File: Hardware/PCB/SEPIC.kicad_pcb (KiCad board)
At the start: 2 copper layers, 33.6 x 35.9 mm, 27 parts, among them Q1 IRF7807, U1 LM3478MA

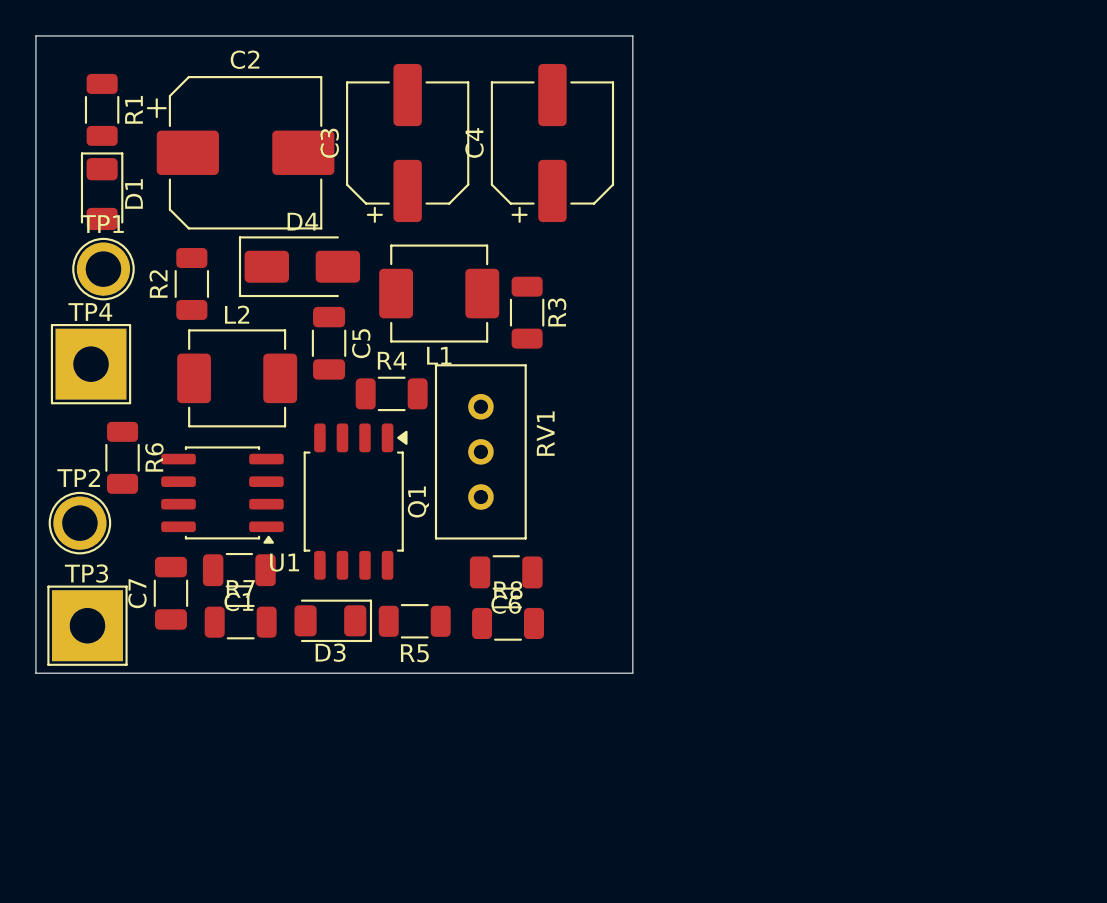
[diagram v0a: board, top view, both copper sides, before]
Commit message: Finished PCB layout
A few minor adjustments still need to be made
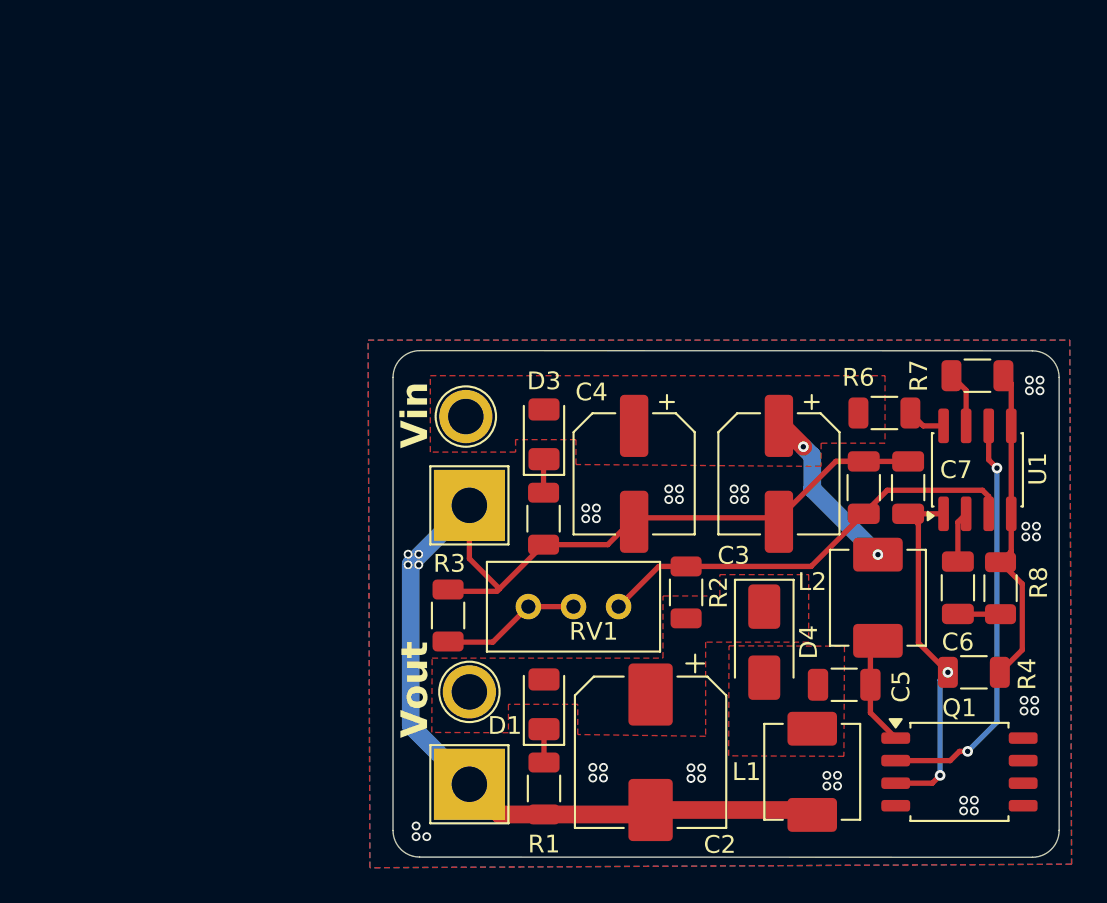
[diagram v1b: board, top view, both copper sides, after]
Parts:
- added G***: LOGO, Logo_footprint:Logo_10_6, B.Cu at (124.3, 65.1)
- added G***: LOGO, Logo_footprint:Logo_15_15, B.Cu at (110.5, 65.2)
- moved R1 45.6 mm to (99.9, 75.8), turned to 90 degrees
- moved R7 43.7 mm to (124.3, 52.6), turned to 180 degrees
- moved R6 43.0 mm to (119.1, 54.7), turned to 180 degrees
- moved U1 42.5 mm to (124.3, 57.9), turned to 90 degrees
- moved C7 41.9 mm to (120.4, 58.9), turned to -90 degrees
- moved C2 40.7 mm to (105.9, 73.8), turned to -90 degrees
- moved L2 38.1 mm to (118.7, 65.1), turned to -90 degrees
- moved D1 38.0 mm to (99.9, 71.1), turned to 90 degrees
- moved Q1 37.3 mm to (123.3, 74.9), turned to 0 degrees
- moved R4 36.3 mm to (124.1, 69.3)
- moved C1 35.5 mm to (117.9, 58.9), turned to -90 degrees
- moved C5 34.8 mm to (116.8, 70.0), turned to 0 degrees
- moved L1 34.1 mm to (115.0, 74.9), turned to 90 degrees
- moved D4 33.5 mm to (112.3, 67.6), turned to -90 degrees
- moved R2 32.8 mm to (107.9, 64.8), turned to -90 degrees
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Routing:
- net GND: track 0.00 -> 92.7 mm, vias 0 -> 47
- net /Feedback: track 0.00 -> 24.7 mm
- net /DR: track 0.00 -> 23.5 mm, vias 0 -> 2
- net /Isen: track 0.00 -> 20.5 mm, vias 0 -> 2
- net Vin: track 0.00 -> 9.77 mm, vias 0 -> 2
- net Net-(R3-Pad2): track 0.00 -> 7.91 mm
- net Net-(Q1-D): track 0.00 -> 6.24 mm
- net Net-(U1-FA/SD): track 0.00 -> 3.17 mm
- net Net-(U1-COMP): track 0.00 -> 2.88 mm
- net Net-(C6-Pad1): track 0.00 -> 2.41 mm
- net Net-(U1-V_{IN}): track 0.00 -> 2.17 mm
- net Net-(D3-K): track 0.00 -> 1.90 mm
- net Net-(D1-K): track 0.00 -> 1.88 mm
- added copper zone on B.Cu, net GND
- added copper zone on F.Cu, net GND
- added copper zone on F.Cu, net Net-(D4-A)
- added copper zone on F.Cu, net Vin
- added copper zone on F.Cu, net Vout
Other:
- board size 33.6 x 35.9 mm -> 37.5 x 28.5 mm
- board text added: "Boost/Buck DC/DC converter |10/10/2026|"
- board text added: "Vin"
- board text added: "Vin : 3-20 V Vout : 3-20 V Max I : 3 A const."
- board text added: "Vout"
